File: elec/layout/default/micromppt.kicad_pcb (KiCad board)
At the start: 2 copper layers, 25.7 x 15.1 mm, 20 parts, among them U5 10µF ±10% 10V X5R, U6 10kΩ ±1% 62.5mW

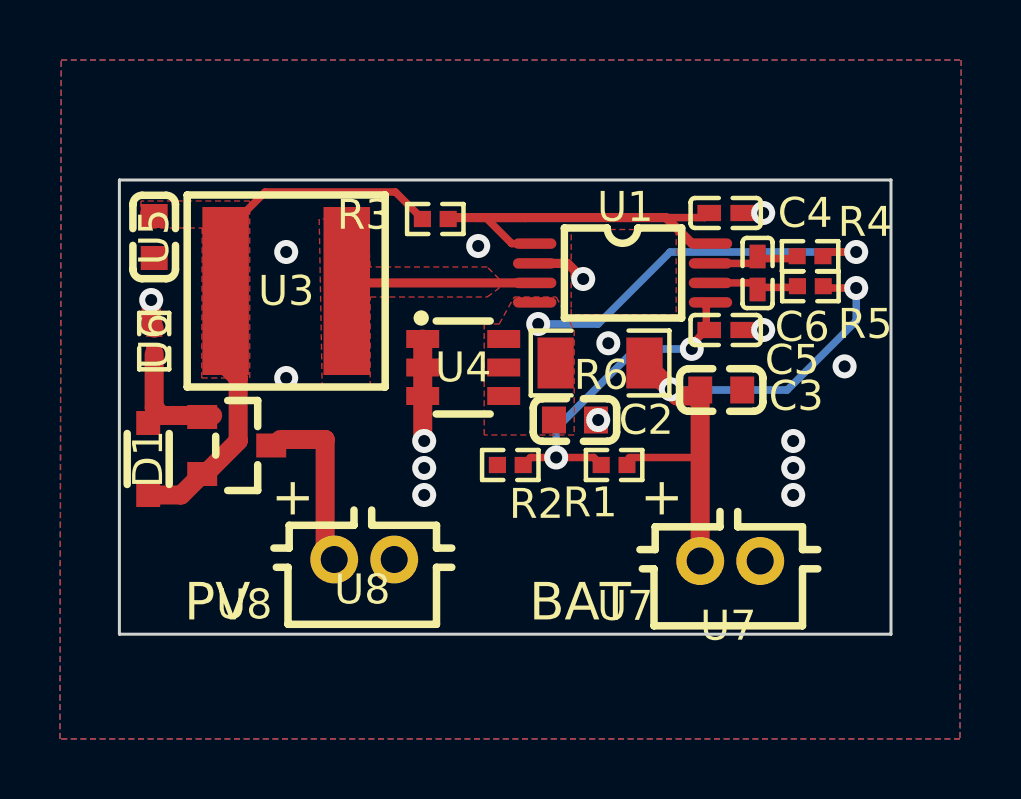
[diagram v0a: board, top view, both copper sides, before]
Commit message: init
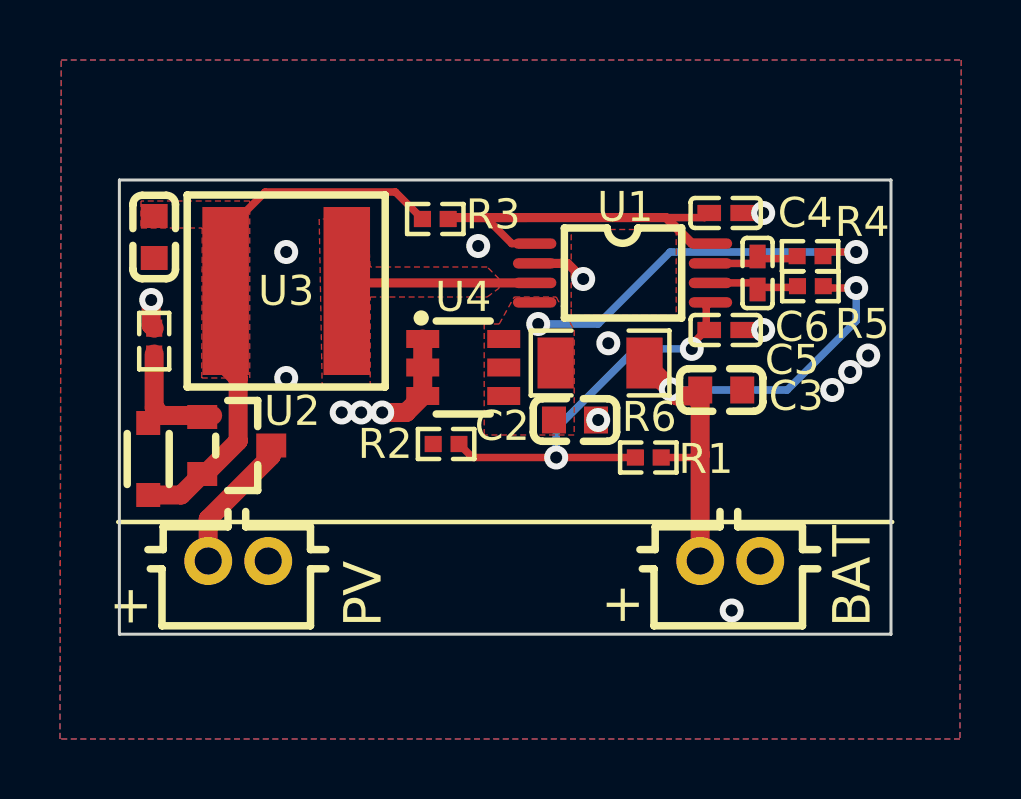
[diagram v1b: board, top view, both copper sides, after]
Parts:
- moved U8 4.20 mm to (70.4, 55.7)
- moved R2 2.25 mm to (77.3, 51.8)
- moved R1 1.17 mm to (84.1, 52.2)
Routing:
- net VCTRL: track 11.2 -> 14.5 mm
- net D: track 5.62 -> 4.72 mm
- net hv: track 19.4 -> 18.5 mm
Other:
- board text removed: "{{GITHASH}}"
